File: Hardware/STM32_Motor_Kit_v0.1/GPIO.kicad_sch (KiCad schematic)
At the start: 1 part, among them J6 Conn_02x09_Odd_Even

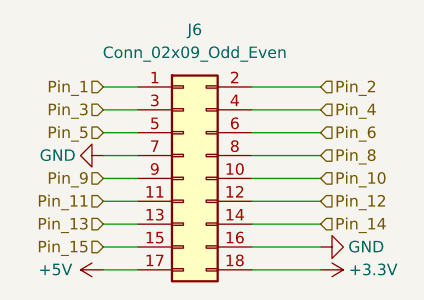
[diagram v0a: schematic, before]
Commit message: 12.01.2025
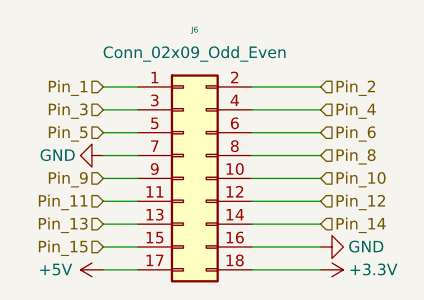
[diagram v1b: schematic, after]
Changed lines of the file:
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@@
 			(effects
 				(font
-					(size 1.27 1.27)
+					(face "Arial")
+					(size 0.635 0.635)
 				)
 				(hide yes)
@@
 			(effects
 				(font
-					(size 1.27 1.27)
+					(face "Arial")
+					(size 0.635 0.635)
 				)
 				(hide yes)
@@
 			(effects
 				(font
-					(size 1.27 1.27)
+					(face "Arial")
+					(size 0.635 0.635)
 				)
 				(hide yes)
@@
 			(effects
 				(font
-					(size 1.27 1.27)
+					(face "Arial")
+					(size 0.635 0.635)
 				)
 			)
@@
 			(effects
 				(font
-					(size 1.27 1.27)
-				)
-				(hide yes)
+					(face "Arial")
+					(size 0.635 0.635)
+				)
+				(hide yes)
